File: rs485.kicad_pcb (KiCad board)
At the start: 2 copper layers, 46.2 x 39.9 mm, 4 parts, among them J1 Conn_01x12_Pin, J3 Conn_01x12_Pin, U2 SN74CB3Q3384APW

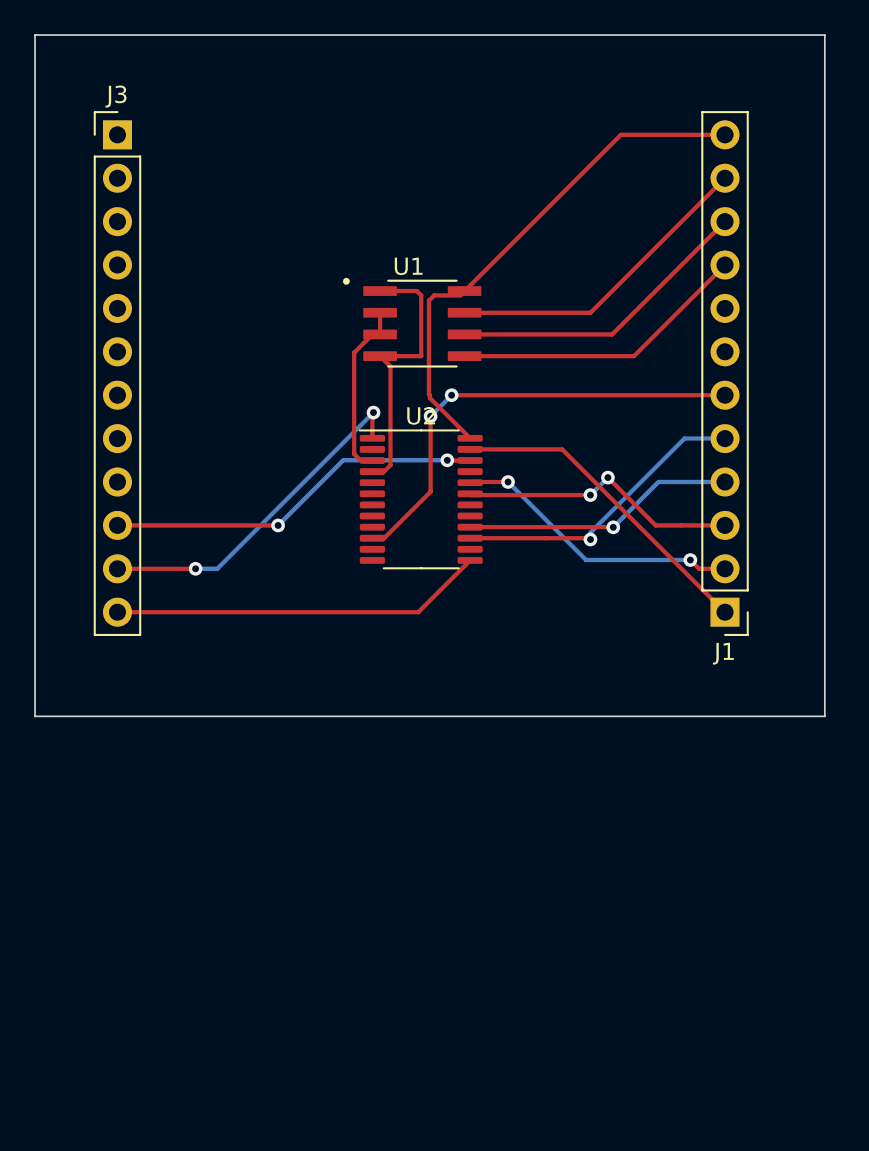
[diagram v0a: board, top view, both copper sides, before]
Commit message: pcb ok.
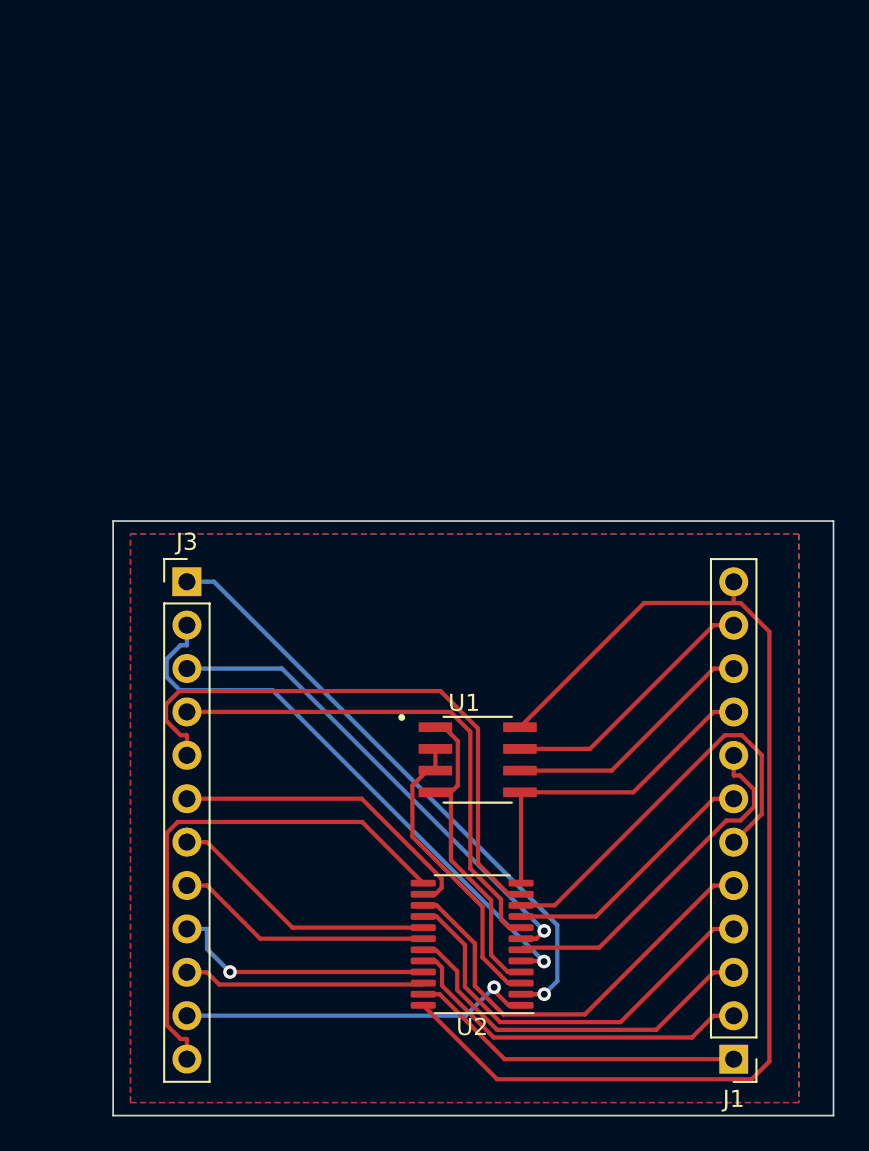
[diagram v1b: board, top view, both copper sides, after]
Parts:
- moved J3 26.5 mm to (133.6, 97.3)
- moved U2 26.2 mm to (150.3, 118.5), turned to 180 degrees
- moved J1 26.2 mm to (165.6, 125.2)
- moved U1 25.7 mm to (150.6, 107.7)
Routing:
- net VCC: track 30.4 -> 67.2 mm
- net Net-(J3-Pin_1): track 0.00 -> 35.7 mm, vias 0 -> 1
- net Net-(J3-Pin_5): track 0.00 -> 34.4 mm
- net Net-(J3-Pin_2): track 0.00 -> 34.1 mm, vias 0 -> 1
- net Net-(J3-Pin_4): track 0.00 -> 30.2 mm
- net Net-(J3-Pin_3): track 0.00 -> 28.8 mm, vias 0 -> 1
- net Net-(J1-Pin_8): track 0.00 -> 20.8 mm
- net Net-(J3-Pin_6): track 0.00 -> 18.6 mm
- net Net-(J3-Pin_7): track 0.00 -> 15.9 mm
- net Net-(J3-Pin_9): track 0.00 -> 15.6 mm, vias 0 -> 1
- net Net-(J1-Pin_7): track 0.00 -> 15.3 mm
- net Net-(J3-Pin_8): track 0.00 -> 15.1 mm
- net Net-(J3-Pin_12): track 21.9 -> 30.7 mm
- net Net-(J1-Pin_4): track 16.0 -> 24.4 mm, vias 1 -> 0
- net Net-(J3-Pin_10): track 22.2 -> 14.2 mm, vias 2 -> 0
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- added copper zone on B.Cu, net GND
- added copper zone on F.Cu, net GND
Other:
- board size 46.2 x 39.9 mm -> 42.2 x 34.8 mm
